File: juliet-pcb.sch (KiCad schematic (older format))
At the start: 94 parts, among them SW0 KEYSW, SW1 KEYSW, SW10 KEYSW, SW11 KEYSW, SW12 KEYSW, SW13 KEYSW, SW14 KEYSW, SW15 KEYSW, SW16 KEYSW, SW17 KEYSW, SW18 KEYSW, SW19 KEYSW, SW2 KEYSW, SW20 KEYSW, SW21 KEYSW, SW22 KEYSW, SW23 KEYSW, SW24 KEYSW, SW25 KEYSW, SW26 KEYSW, SW27 KEYSW, SW28 KEYSW, SW29 KEYSW, SW3 KEYSW, SW30 KEYSW, SW31 KEYSW, SW32 KEYSW, SW33 KEYSW, SW34 KEYSW, SW35 KEYSW, SW36 KEYSW, SW37 KEYSW, SW38 KEYSW, SW39 KEYSW, SW4 KEYSW, SW40 KEYSW, SW41 KEYSW, SW42 KEYSW, SW43 KEYSW, SW44 KEYSW, SW45 KEYSW, SW46 KEYSW, SW47 KEYSW, SW5 KEYSW, SW6 KEYSW, SW7 KEYSW, SW8 KEYSW, SW9 KEYSW, U1 Pro_Micro

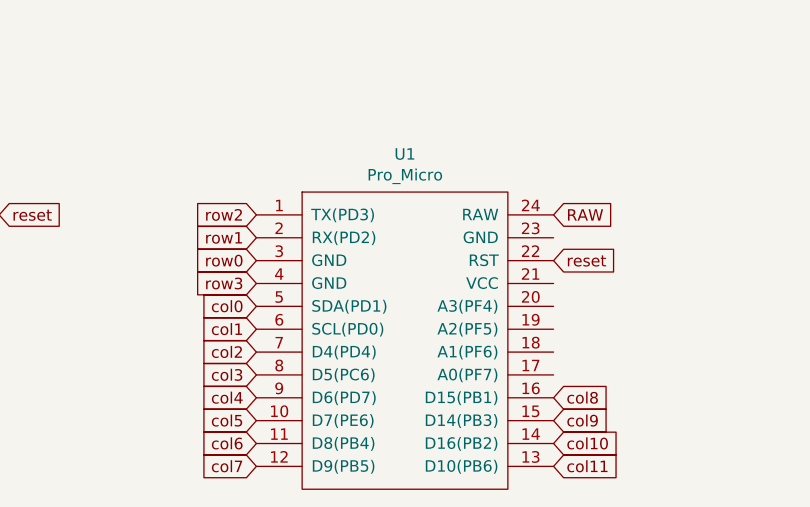
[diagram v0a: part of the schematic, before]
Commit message: lol fixed
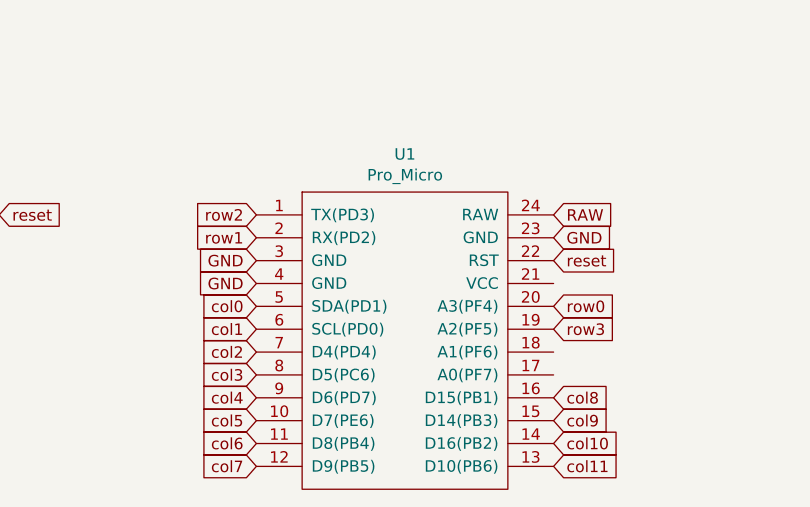
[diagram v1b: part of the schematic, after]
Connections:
- net GND: now also U1.23 (GND), U1.3 (GND), U1.4 (GND)
- net row0: now also U1.20 (A3(PF4)); no longer U1.3 (GND)
- net row3: now also U1.19 (A2(PF5)); no longer U1.4 (GND)
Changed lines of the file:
@@
 Text GLabel 7200 4500 2    50   Input ~ 0
 reset
-Text GLabel 5900 4500 0    50   Input ~ 0
+Text GLabel 7200 4700 2    50   Input ~ 0
 row0
 Text GLabel 5900 4400 0    50   Input ~ 0
@@
 Text GLabel 5900 4300 0    50   Input ~ 0
 row2
-Text GLabel 5900 4600 0    50   Input ~ 0
+Text GLabel 7200 4800 2    50   Input ~ 0
 row3
 Text GLabel 5900 4700 0    50   Input ~ 0
@@
 Text GLabel 7200 4300 2    50   Input ~ 0
 RAW
+Text GLabel 5900 4500 0    50   Input ~ 0
+GND
+Text GLabel 5900 4600 0    50   Input ~ 0
+GND
+Text GLabel 7200 4400 2    50   Input ~ 0
+GND
 $EndSCHEMATC
